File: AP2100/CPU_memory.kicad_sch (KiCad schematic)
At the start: 1 part, among them U1 LS1043ASE7KQB

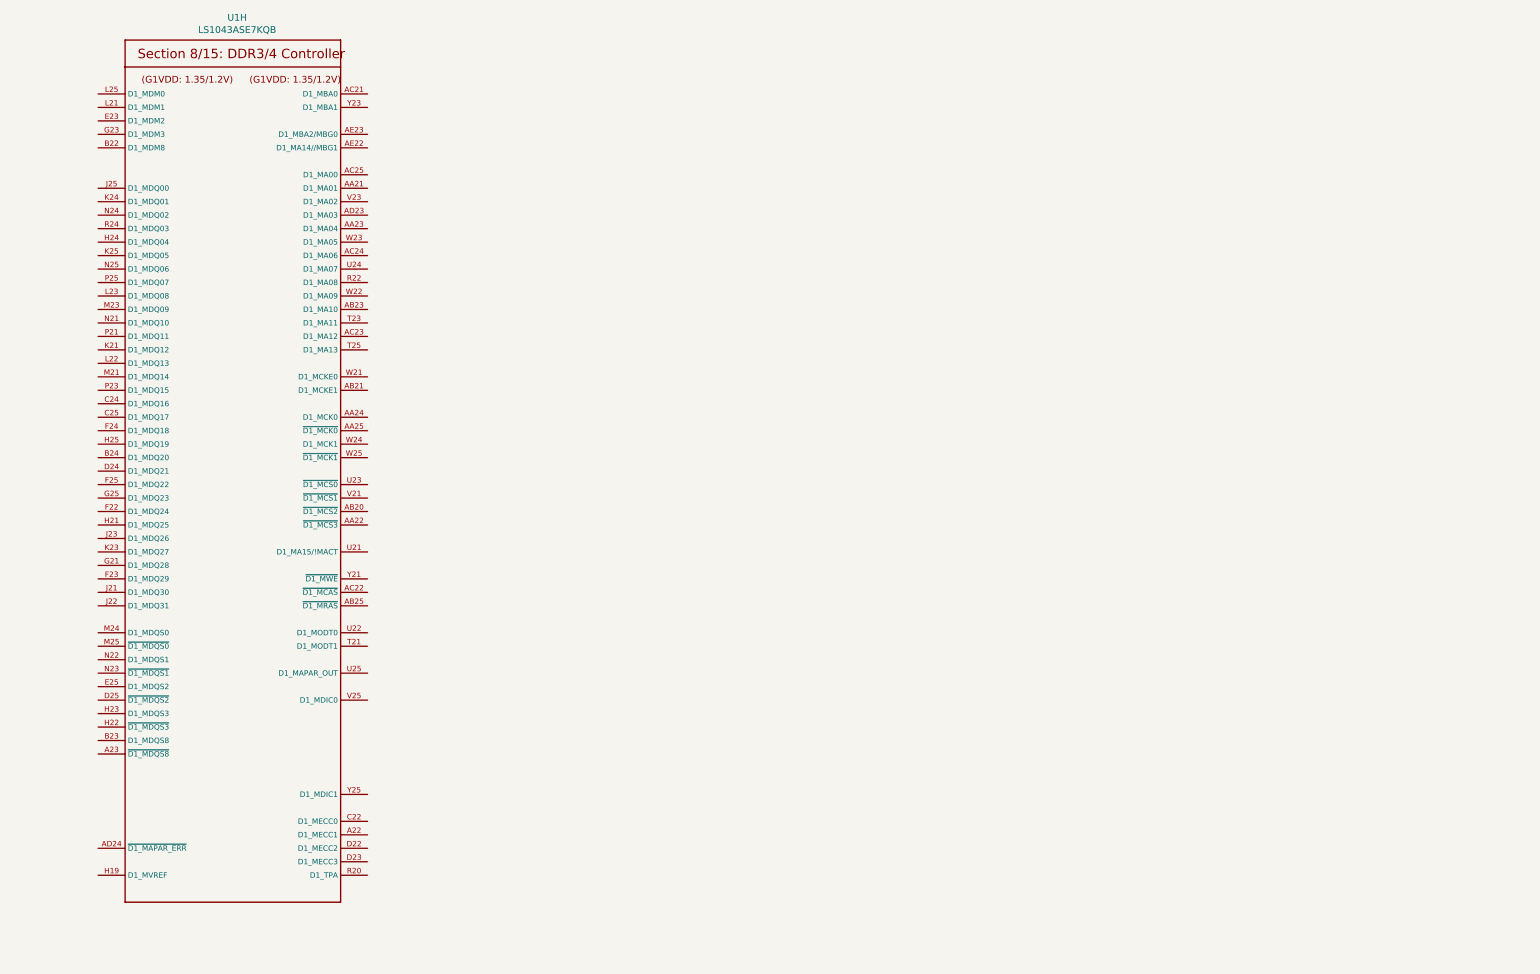
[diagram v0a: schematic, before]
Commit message: More work on memory
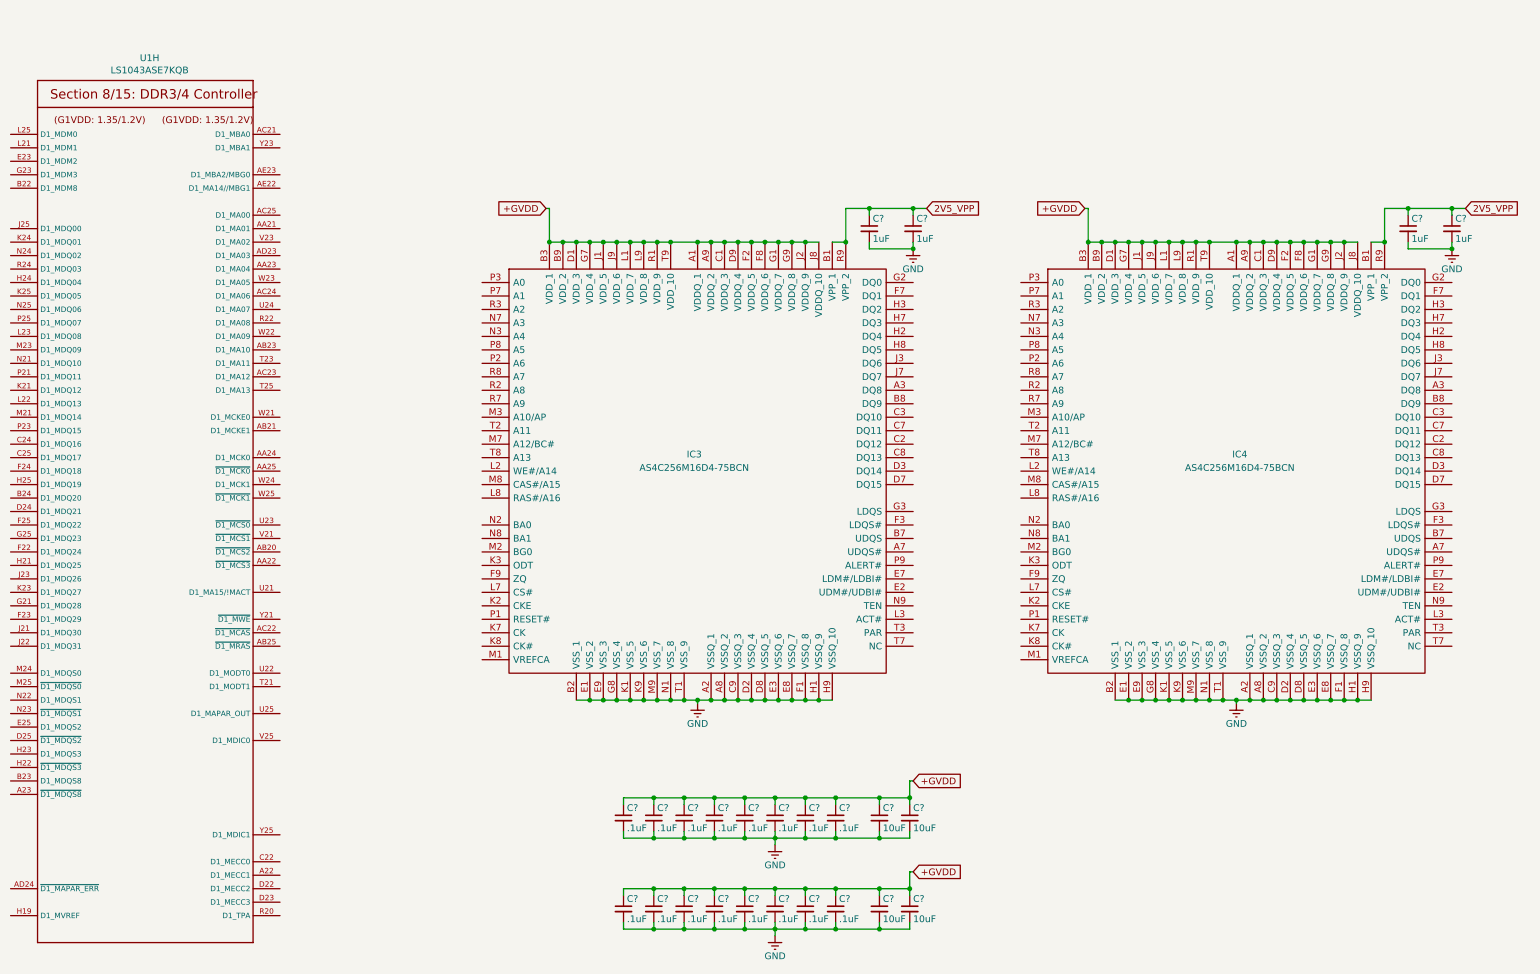
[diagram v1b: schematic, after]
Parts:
- added C? (x4): 1uF, Capacitor_SMD:C_0402_1005Metric, symbol Device:C_Small
- added C? (x16): .1uF, Capacitor_SMD:C_0402_1005Metric, symbol Device:C_Small
- added C? (x4): 10uF, Capacitor_SMD:C_0805_2012Metric, symbol Device:C_Small
- added IC3, IC4: AS4C256M16D4-75BCN, Scott:BGA96C80P9X16_750X1350X120, symbol Scott:AS4C256M16D4
- U1: MFR - -> (none)
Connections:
- new net +GVDD: C?.1, C?.1, C?.1, C?.1, C?.1, C?.1, C?.1, C?.1, C?.1, C?.1, C?.1, C?.1, C?.1, C?.1, C?.1, C?.1, C?.1, C?.1, C?.1, C?.1, IC3.A1 (VDDQ_1), IC3.A9 (VDDQ_2), IC3.B3 (VDD_1), IC3.B9 (VDD_2), IC3.C1 (VDDQ_3), IC3.D1 (VDD_3), IC3.D9 (VDDQ_4), IC3.F2 (VDDQ_5), IC3.F8 (VDDQ_6), IC3.G1 (VDDQ_7), IC3.G7 (VDD_4), IC3.G9 (VDDQ_8), IC3.J1 (VDD_5), IC3.J2 (VDDQ_9), IC3.J8 (VDDQ_10), IC3.J9 (VDD_6), IC3.L1 (VDD_7), IC3.L9 (VDD_8), IC3.R1 (VDD_9), IC3.T9 (VDD_10), IC4.A1 (VDDQ_1), IC4.A9 (VDDQ_2), IC4.B3 (VDD_1), IC4.B9 (VDD_2), IC4.C1 (VDDQ_3), IC4.D1 (VDD_3), IC4.D9 (VDDQ_4), IC4.F2 (VDDQ_5), IC4.F8 (VDDQ_6), IC4.G1 (VDDQ_7), IC4.G7 (VDD_4), IC4.G9 (VDDQ_8), IC4.J1 (VDD_5), IC4.J2 (VDDQ_9), IC4.J8 (VDDQ_10), IC4.J9 (VDD_6), IC4.L1 (VDD_7), IC4.L9 (VDD_8), IC4.R1 (VDD_9), IC4.T9 (VDD_10)
- new net 2V5_VPP: C?.1, C?.1, C?.1, C?.1, IC3.B1 (VPP_1), IC3.R9 (VPP_2), IC4.B1 (VPP_1), IC4.R9 (VPP_2)
- new net GND: C?.2, C?.2, C?.2, C?.2, C?.2, C?.2, C?.2, C?.2, C?.2, C?.2, C?.2, C?.2, C?.2, C?.2, C?.2, C?.2, C?.2, C?.2, C?.2, C?.2, C?.2, C?.2, C?.2, C?.2, IC3.A2 (VSSQ_1), IC3.A8 (VSSQ_2), IC3.B2 (VSS_1), IC3.C9 (VSSQ_3), IC3.D2 (VSSQ_4), IC3.D8 (VSSQ_5), IC3.E1 (VSS_2), IC3.E3 (VSSQ_6), IC3.E8 (VSSQ_7), IC3.E9 (VSS_3), IC3.F1 (VSSQ_8), IC3.G8 (VSS_4), IC3.H1 (VSSQ_9), IC3.H9 (VSSQ_10), IC3.K1 (VSS_5), IC3.K9 (VSS_6), IC3.M9 (VSS_7), IC3.N1 (VSS_8), IC3.T1 (VSS_9), IC4.A2 (VSSQ_1), IC4.A8 (VSSQ_2), IC4.B2 (VSS_1), IC4.C9 (VSSQ_3), IC4.D2 (VSSQ_4), IC4.D8 (VSSQ_5), IC4.E1 (VSS_2), IC4.E3 (VSSQ_6), IC4.E8 (VSSQ_7), IC4.E9 (VSS_3), IC4.F1 (VSSQ_8), IC4.G8 (VSS_4), IC4.H1 (VSSQ_9), IC4.H9 (VSSQ_10), IC4.K1 (VSS_5), IC4.K9 (VSS_6), IC4.M9 (VSS_7), IC4.N1 (VSS_8), IC4.T1 (VSS_9)
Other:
- moved on the sheet: U1H
